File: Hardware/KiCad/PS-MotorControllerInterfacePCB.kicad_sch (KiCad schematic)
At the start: 50 parts, among them J1 PWR board, J2 CAN board out, J3 CAN board in, J4 Candapter, J5 53307-2471, J6 CAN board -> mppt +moco, J7 CAN mppts + moco -> board, J8 PWR Moco

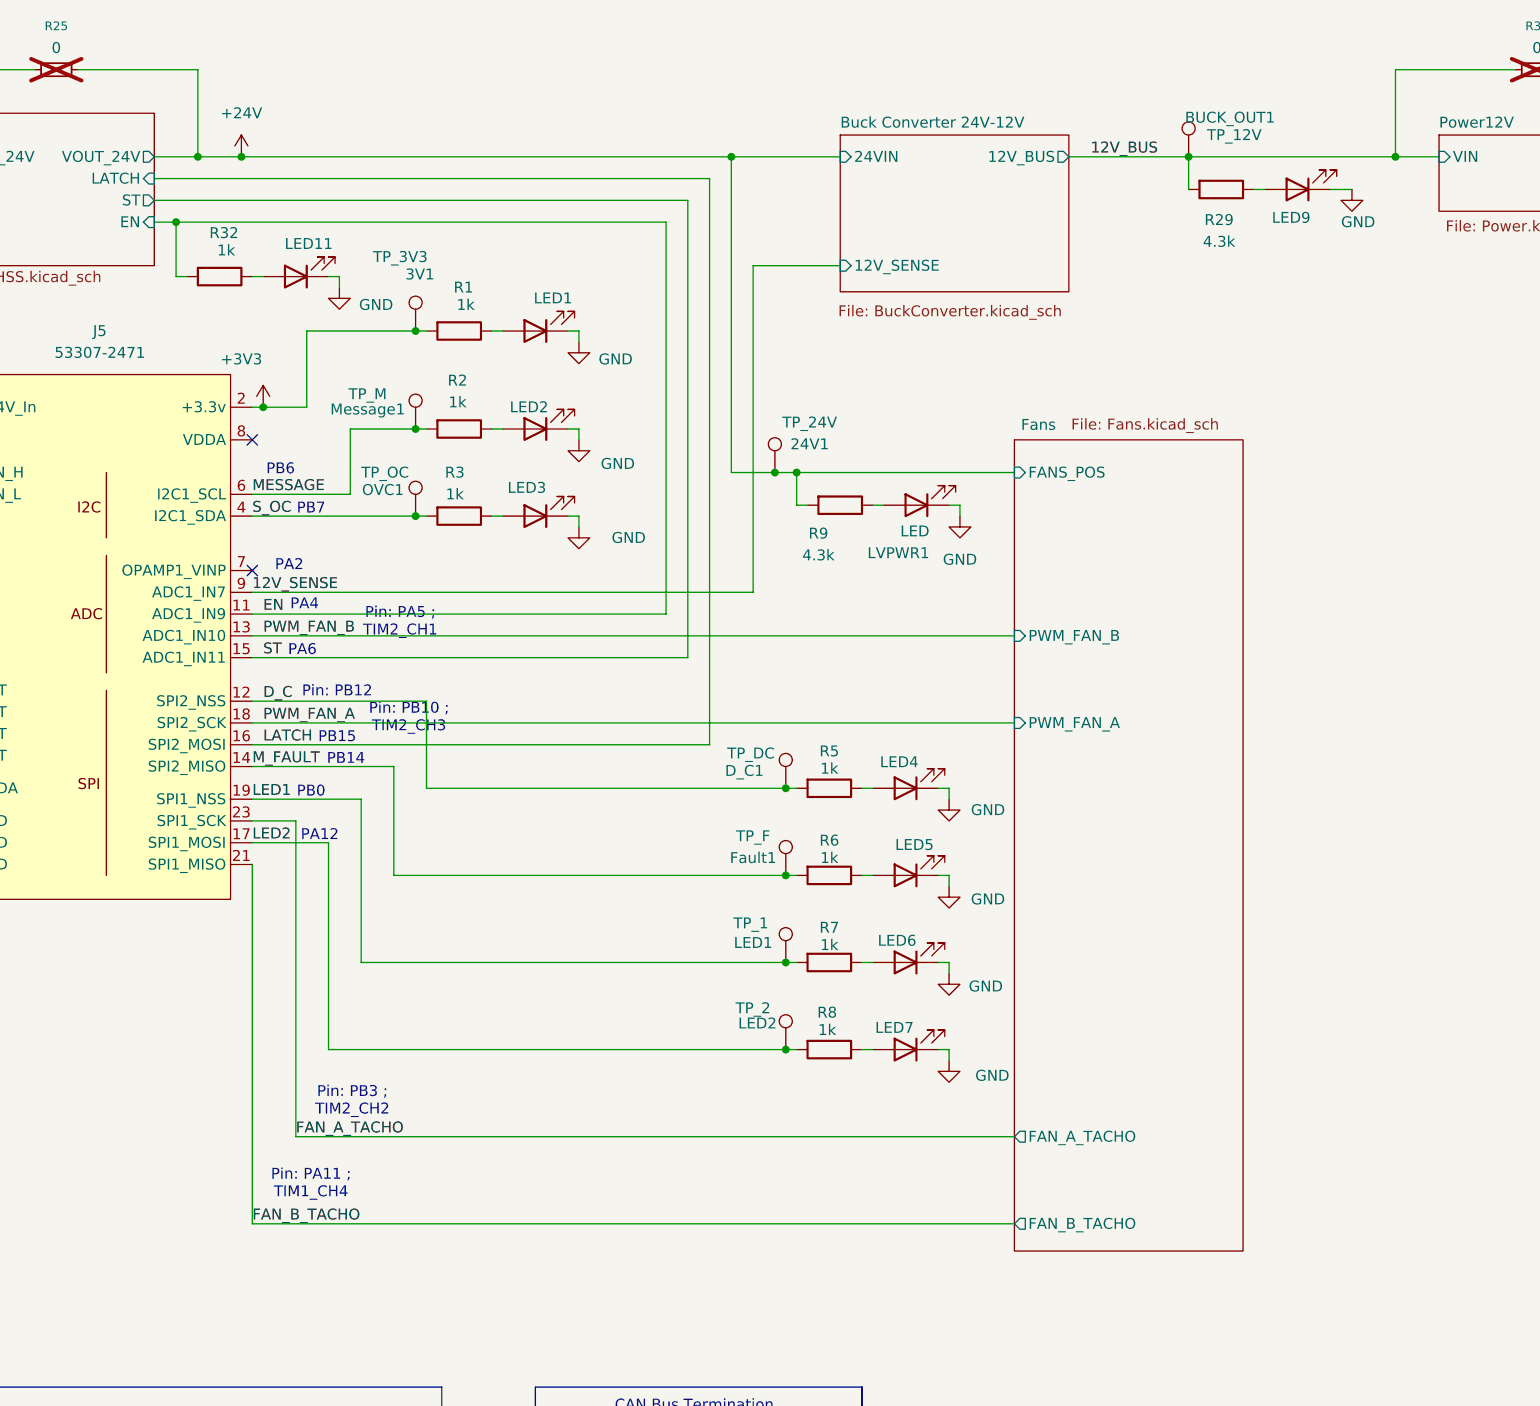
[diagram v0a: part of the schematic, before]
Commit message: changes
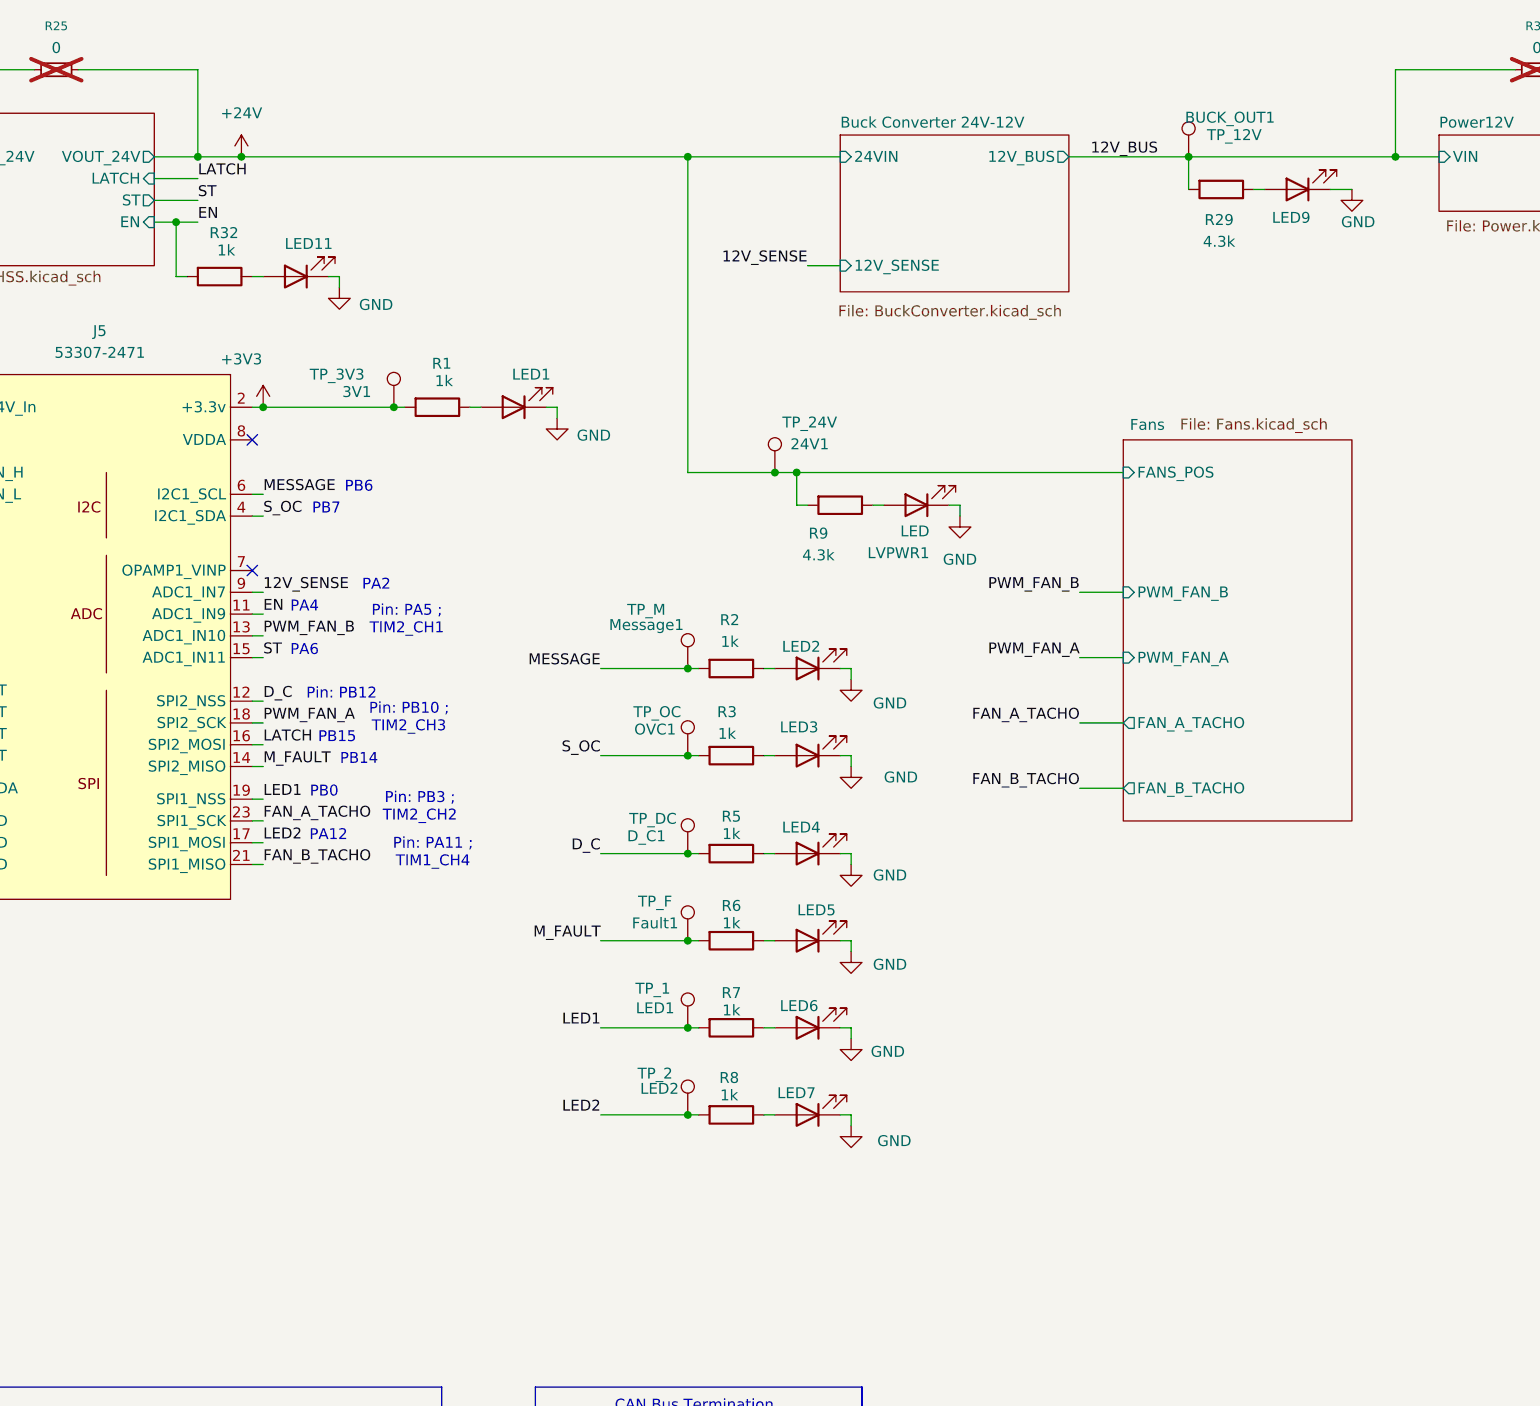
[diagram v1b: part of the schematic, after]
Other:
- moved on the sheet: 3V1, D_C1, Fault1, LED1, LED2, LED3, LED4, LED5, LED6, LED7, Message1, OVC1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
